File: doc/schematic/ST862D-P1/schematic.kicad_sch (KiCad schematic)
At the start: 2 parts, among them J1 AC-OUT, J2 AC-IN

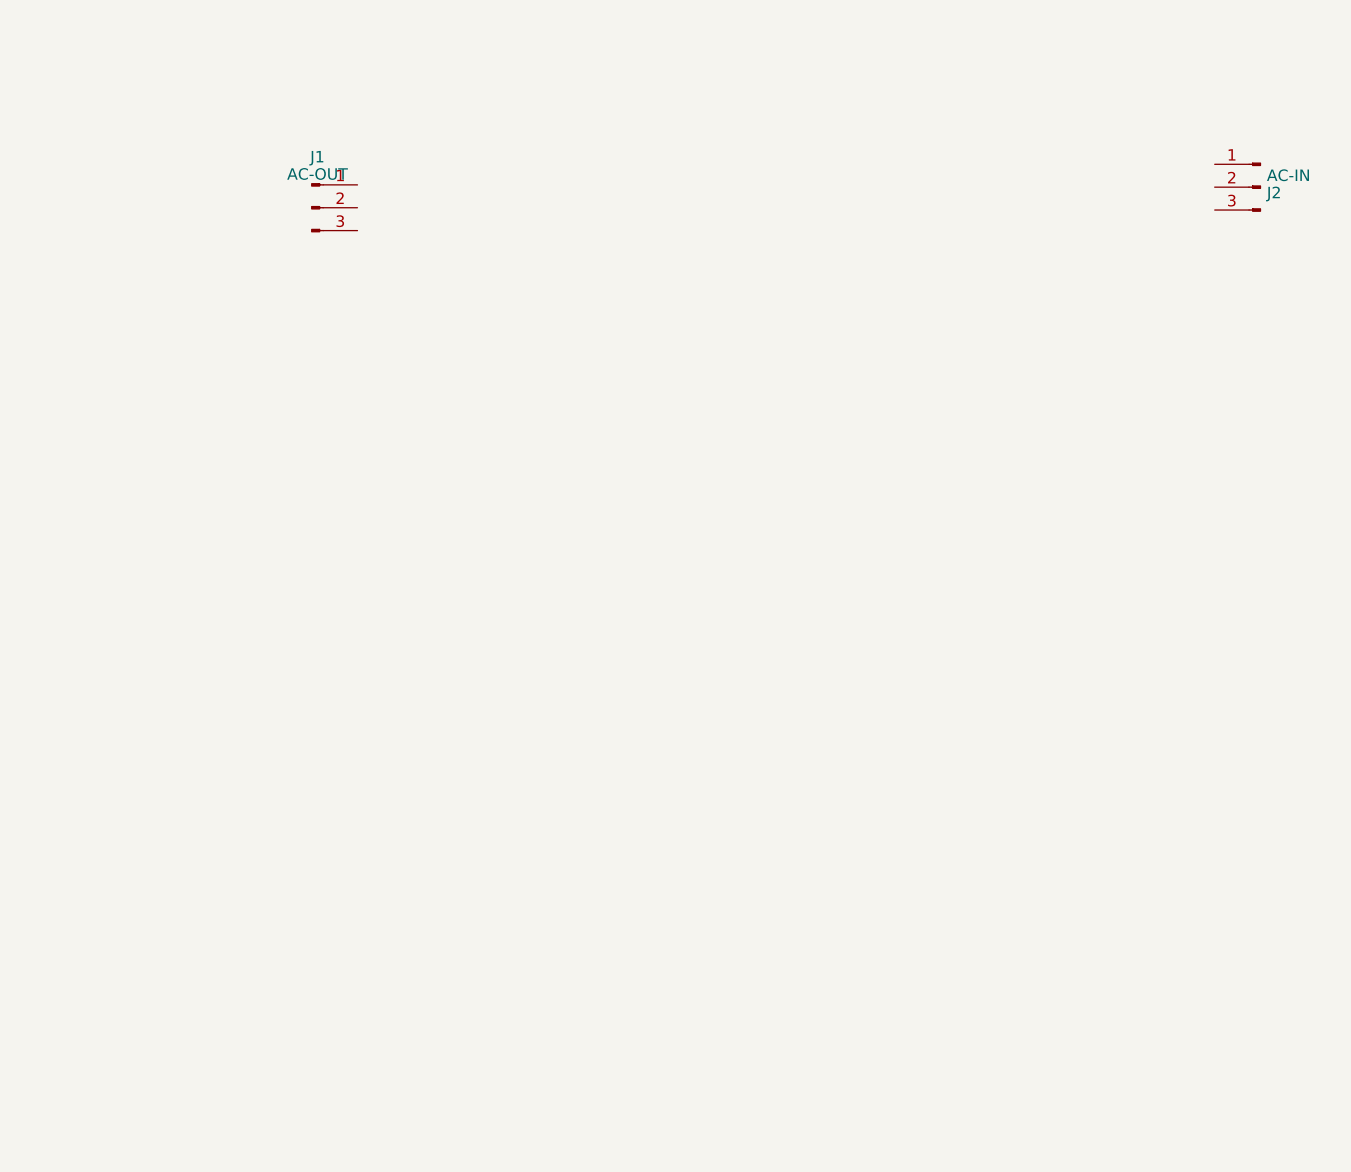
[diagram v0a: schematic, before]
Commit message: Update Schematics
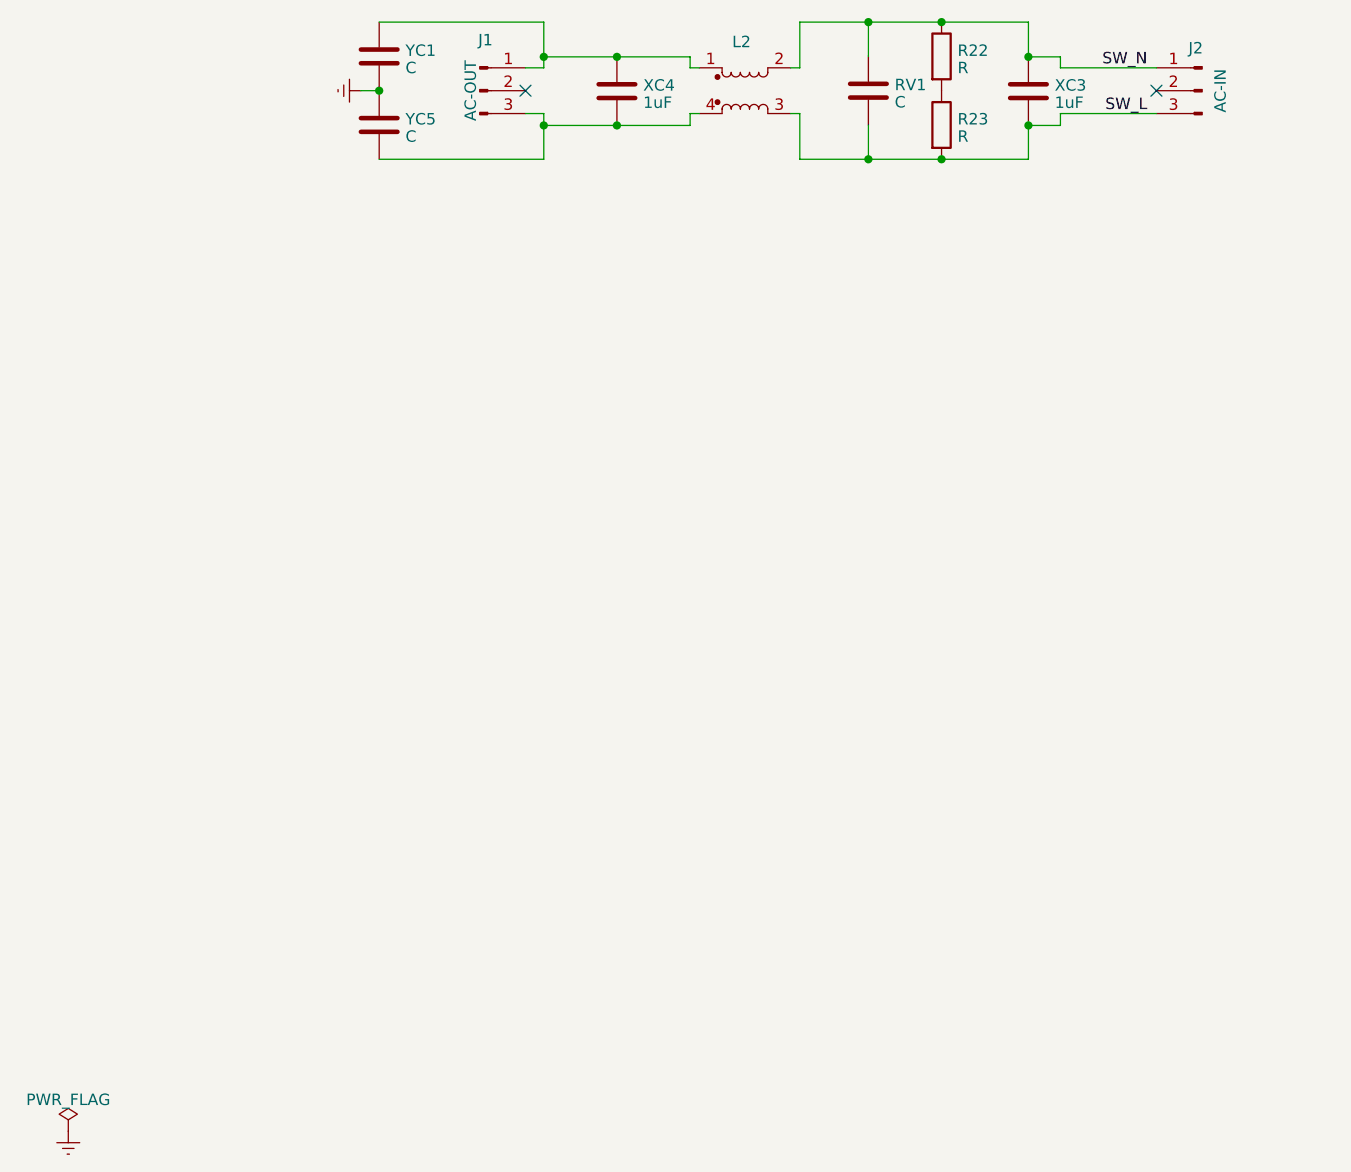
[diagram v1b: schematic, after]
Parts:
- added L2: ~, symbol Device:L_Coupled_1243
- added R22, R23: R, symbol Device:R
- added RV1, YC1, YC5: C, symbol Device:C
- added XC3, XC4: 1uF, symbol Device:C
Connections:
- net at J1.1 (Pin_1): now also L2.1, XC4.1, YC1.1
- net at J1.3 (Pin_3): now also L2.4, XC4.2, YC5.2
- net SW_N: now reaches J2.1 (Pin_1)
- net SW_N: now also L2.2, R22.1, RV1.1, XC3.1
- net SW_L: now reaches J2.3 (Pin_3)
- net SW_L: now also L2.3, R23.2, RV1.2, XC3.2
- new net: R22.2, R23.1
- new net Earth: YC1.2, YC5.1
- no-connect marks 0 -> 2
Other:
- moved on the sheet: J1, J2

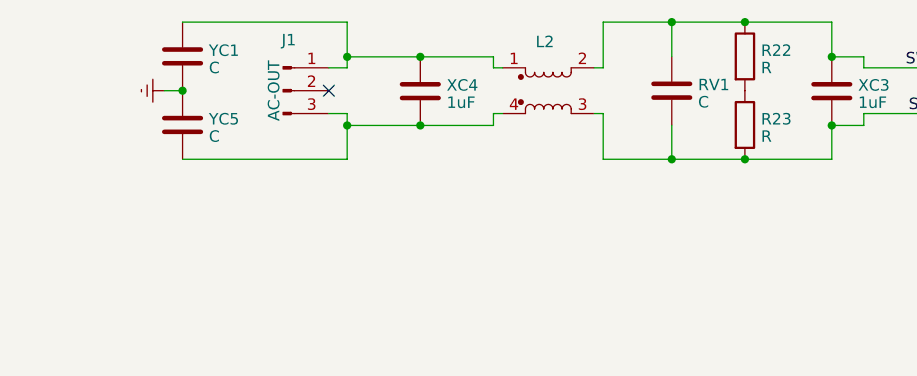
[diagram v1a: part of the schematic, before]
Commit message: Update Schematic
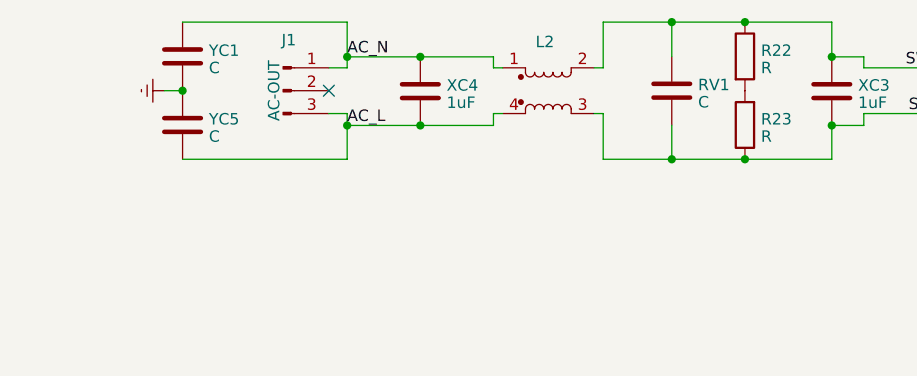
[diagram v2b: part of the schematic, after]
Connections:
- net Earth: now also YC5.2; no longer YC5.1
- net SW_L: now also R23.1; no longer R23.2
- net AC_N: now reaches J1.1 (Pin_1), L2.1, XC4.1, YC1.1
- net AC_L: now reaches J1.3 (Pin_3), L2.4, XC4.2
- net AC_L: now also YC5.1; no longer YC5.2
- net at R22.2: now also R23.2; no longer R23.1
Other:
- moved on the sheet: R23, YC5
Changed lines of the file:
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@@
     (company "4Source")
   )
+  (junction (at 59.944 72.3392) (diameter 0) (color 0 0 0 0)
+  )
   (junction (at 78.232 68.58) (diameter 0) (color 0 0 0 0)
   )
@@
   (junction (at 132.08 76.2) (diameter 0) (color 0 0 0 0)
   )
+  (junction (at 122.428 79.9592) (diameter 0) (color 0 0 0 0)
+  )
   (junction (at 86.36 76.2) (diameter 0) (color 0 0 0 0)
   )
   (junction (at 114.3 79.9592) (diameter 0) (color 0 0 0 0)
   )
-  (junction (at 59.944 72.3392) (diameter 0) (color 0 0 0 0)
-  )
   (junction (at 86.36 68.58) (diameter 0) (color 0 0 0 0)
   )
@@
   )
   (junction (at 132.08 68.58) (diameter 0) (color 0 0 0 0)
-  )
-  (junction (at 122.428 79.9592) (diameter 0) (color 0 0 0 0)
   )
   (junction (at 78.232 76.2) (diameter 0) (color 0 0 0 0)
@@
     (stroke (width 0) (type default))
   )
+  (wire (pts (xy 114.3 79.9592) (xy 122.428 79.9592))
+    (stroke (width 0) (type default))
+  )
+  (wire (pts (xy 78.232 79.9592) (xy 78.232 76.2))
+    (stroke (width 0) (type default))
+  )
+  (wire (pts (xy 59.944 79.9592) (xy 78.232 79.9592))
+    (stroke (width 0) (type default))
+  )
+  (wire (pts (xy 122.428 64.7192) (xy 132.08 64.7192))
+    (stroke (width 0) (type default))
+  )
+  (wire (pts (xy 95.504 69.7992) (xy 94.488 69.7992))
+    (stroke (width 0) (type default))
+  )
+  (wire (pts (xy 78.232 74.8792) (xy 78.232 76.2))
+    (stroke (width 0) (type default))
+  )
+  (wire (pts (xy 78.232 64.7192) (xy 78.232 68.58))
+    (stroke (width 0) (type default))
+  )
+  (wire (pts (xy 132.08 64.7192) (xy 132.08 68.58))
+    (stroke (width 0) (type default))
+  )
+  (wire (pts (xy 94.488 69.7992) (xy 94.488 68.58))
+    (stroke (width 0) (type default))
+  )
+  (wire (pts (xy 94.488 74.8792) (xy 94.488 76.2))
+    (stroke (width 0) (type default))
+  )
+  (wire (pts (xy 76.2 74.8792) (xy 78.232 74.8792))
+    (stroke (width 0) (type default))
+  )
+  (wire (pts (xy 106.68 74.8792) (xy 106.68 79.9592))
+    (stroke (width 0) (type default))
+  )
+  (wire (pts (xy 105.664 74.8792) (xy 106.68 74.8792))
+    (stroke (width 0) (type default))
+  )
+  (wire (pts (xy 135.636 76.2) (xy 135.636 74.8792))
+    (stroke (width 0) (type default))
+  )
+  (wire (pts (xy 76.2 69.7992) (xy 78.232 69.7992))
+    (stroke (width 0) (type default))
+  )
+  (wire (pts (xy 94.488 76.2) (xy 86.36 76.2))
+    (stroke (width 0) (type default))
+  )
+  (wire (pts (xy 106.68 79.9592) (xy 114.3 79.9592))
+    (stroke (width 0) (type default))
+  )
+  (wire (pts (xy 114.3 76.1492) (xy 114.3 79.9592))
+    (stroke (width 0) (type default))
+  )
+  (wire (pts (xy 57.912 72.3392) (xy 59.944 72.3392))
+    (stroke (width 0) (type default))
+  )
+  (wire (pts (xy 78.232 68.58) (xy 86.36 68.58))
+    (stroke (width 0) (type default))
+  )
+  (wire (pts (xy 114.3 64.7192) (xy 122.428 64.7192))
+    (stroke (width 0) (type default))
+  )
+  (wire (pts (xy 106.68 64.7192) (xy 114.3 64.7192))
+    (stroke (width 0) (type default))
+  )
+  (wire (pts (xy 105.664 69.7992) (xy 106.68 69.7992))
+    (stroke (width 0) (type default))
+  )
+  (wire (pts (xy 78.232 69.7992) (xy 78.232 68.58))
+    (stroke (width 0) (type default))
+  )
+  (wire (pts (xy 135.636 74.8792) (xy 146.304 74.8792))
+    (stroke (width 0) (type default))
+  )
   (wire (pts (xy 122.428 79.9592) (xy 132.08 79.9592))
     (stroke (width 0) (type default))
   )
-  (wire (pts (xy 78.232 79.9592) (xy 78.232 76.2))
-    (stroke (width 0) (type default))
-  )
-  (wire (pts (xy 59.944 79.9592) (xy 78.232 79.9592))
-    (stroke (width 0) (type default))
-  )
-  (wire (pts (xy 122.428 64.7192) (xy 132.08 64.7192))
-    (stroke (width 0) (type default))
-  )
-  (wire (pts (xy 95.504 69.7992) (xy 94.488 69.7992))
-    (stroke (width 0) (type default))
-  )
-  (wire (pts (xy 78.232 74.8792) (xy 78.232 76.2))
-    (stroke (width 0) (type default))
-  )
-  (wire (pts (xy 78.232 64.7192) (xy 78.232 68.58))
-    (stroke (width 0) (type default))
-  )
-  (wire (pts (xy 132.08 64.7192) (xy 132.08 68.58))
-    (stroke (width 0) (type default))
-  )
-  (wire (pts (xy 94.488 69.7992) (xy 94.488 68.58))
-    (stroke (width 0) (type default))
-  )
-  (wire (pts (xy 94.488 74.8792) (xy 94.488 76.2))
-    (stroke (width 0) (type default))
-  )
-  (wire (pts (xy 76.2 74.8792) (xy 78.232 74.8792))
-    (stroke (width 0) (type default))
-  )
-  (wire (pts (xy 106.68 74.8792) (xy 106.68 79.9592))
-    (stroke (width 0) (type default))
-  )
-  (wire (pts (xy 105.664 74.8792) (xy 106.68 74.8792))
-    (stroke (width 0) (type default))
-  )
-  (wire (pts (xy 135.636 76.2) (xy 135.636 74.8792))
-    (stroke (width 0) (type default))
-  )
-  (wire (pts (xy 76.2 69.7992) (xy 78.232 69.7992))
-    (stroke (width 0) (type default))
-  )
-  (wire (pts (xy 94.488 76.2) (xy 86.36 76.2))
-    (stroke (width 0) (type default))
-  )
-  (wire (pts (xy 106.68 79.9592) (xy 114.3 79.9592))
-    (stroke (width 0) (type default))
-  )
-  (wire (pts (xy 114.3 76.1492) (xy 114.3 79.9592))
-    (stroke (width 0) (type default))
-  )
-  (wire (pts (xy 57.912 72.3392) (xy 59.944 72.3392))
-    (stroke (width 0) (type default))
-  )
-  (wire (pts (xy 78.232 68.58) (xy 86.36 68.58))
-    (stroke (width 0) (type default))
-  )
-  (wire (pts (xy 114.3 64.7192) (xy 122.428 64.7192))
-    (stroke (width 0) (type default))
-  )
-  (wire (pts (xy 106.68 64.7192) (xy 114.3 64.7192))
-    (stroke (width 0) (type default))
-  )
-  (wire (pts (xy 105.664 69.7992) (xy 106.68 69.7992))
-    (stroke (width 0) (type default))
-  )
-  (wire (pts (xy 78.232 69.7992) (xy 78.232 68.58))
-    (stroke (width 0) (type default))
-  )
-  (wire (pts (xy 135.636 74.8792) (xy 146.304 74.8792))
-    (stroke (width 0) (type default))
-  )
   (wire (pts (xy 114.3 68.5292) (xy 114.3 64.7192))
     (stroke (width 0) (type default))
@@
     (stroke (width 0) (type default))
   )
-  (wire (pts (xy 114.3 79.9592) (xy 122.428 79.9592))
-    (stroke (width 0) (type default))
-  )
   (wire (pts (xy 59.944 64.7192) (xy 78.232 64.7192))
     (stroke (width 0) (type default))
@@
   (wire (pts (xy 132.08 68.58) (xy 135.636 68.58))
     (stroke (width 0) (type default))
+  )
+  (label "AC_L" (at 78.232 76.2 0) (fields_autoplaced)
+    (effects (font (size 1.27 1.27)) (justify left bottom))
   )
   (label "SW_L" (at 145.288 74.8792 180) (fields_autoplaced)
@@
     (effects (font (size 1.27 1.27)) (justify right bottom))
   )
+  (label "AC_N" (at 78.232 68.58 0) (fields_autoplaced)
+    (effects (font (size 1.27 1.27)) (justify left bottom))
+  )
   (symbol (lib_id "Device:C") (at 114.3 72.3392 0) (unit 1)
     (in_bom yes) (on_board yes) (dnp no) (fields_autoplaced)
@@
     )
   )
-  (symbol (lib_id "Device:C") (at 59.944 76.1492 0) (unit 1)
+  (symbol (lib_id "Device:C") (at 59.944 76.1492 180) (unit 1)
     (in_bom yes) (on_board yes) (dnp no) (fields_autoplaced)
     (property "Reference" "YC5" (at 62.865 75.5055 0)
-      (effects (font (size 1.27 1.27)) (justify left))
+      (effects (font (size 1.27 1.27)) (justify right))
     )
     (property "Value" "C" (at 62.865 77.4265 0)
-      (effects (font (size 1.27 1.27)) (justify left))
-    )
-    (property "Footprint" "" (at 60.9092 79.9592 0)
+      (effects (font (size 1.27 1.27)) (justify right))
+    )
+    (property "Footprint" "" (at 58.9788 72.3392 0)
       (effects (font (size 1.27 1.27)) hide)
     )
@@
     )
   )
-  (symbol (lib_id "Device:R") (at 122.428 76.1492 0) (unit 1)
+  (symbol (lib_id "Device:R") (at 122.428 76.1492 180) (unit 1)
     (in_bom yes) (on_board yes) (dnp no) (fields_autoplaced)
     (property "Reference" "R23" (at 124.206 75.5055 0)
-      (effects (font (size 1.27 1.27)) (justify left))
+      (effects (font (size 1.27 1.27)) (justify right))
     )
     (property "Value" "R" (at 124.206 77.4265 0)
-      (effects (font (size 1.27 1.27)) (justify left))
-    )
-    (property "Footprint" "" (at 120.65 76.1492 90)
-      (effects (font (size 1.27 1.27)) hide)
-    )
+      (effects (font (size 1.27 1.27)) (justify right))
+    )
+    (property "Footprint" "" (at 124.206 76.1492 90)
+      (effects (font (size 1.27 1.27)) hide)
+    )
